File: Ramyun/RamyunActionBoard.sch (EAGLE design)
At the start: 84 parts, among them Q1 BC817-16LT1SMD, Q2 BC817-16LT1SMD, Q3 NVF6P02, U1 MAX31856_ADAFRUIT, U10 PVN012PBF, U11 PVN012PBF, U12 PVN012PBF, U13 PVN012PBF, U2 MAX31856_ADAFRUIT, U3 NL17SZ17DFT, U4 GPS_ADAFRUIT, U5 BUZZER, U6 PVN012PBF, U7 PVN012PBF, U8 PVN012PBF, U9 PVN012PBF, X1 5267-03, X10 5267-02, X11 5267-02, X12 5267-02, X13 5267-02, X14 5267-02, X15 5267-02, X16 5267-02, X2 5267-03, X3 5267-03, X4 USB+SHIELD, X5 5267-02, X6 5267-02, X7 5267-02, X8 5267-02, X9 5267-02

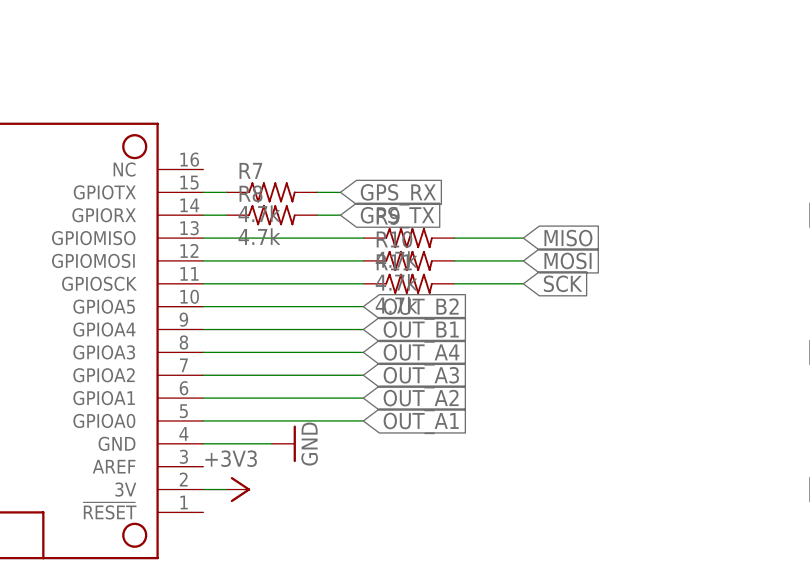
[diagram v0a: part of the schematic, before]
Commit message: value changed
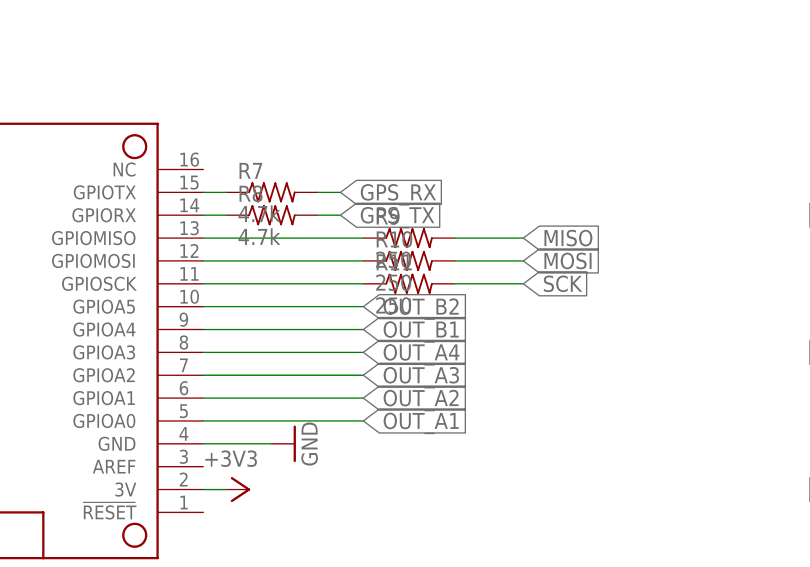
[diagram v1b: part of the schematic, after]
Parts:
- R10, R11, R9: value 4.7k -> 250
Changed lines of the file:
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@@
 <part name="GND_EXT25" library="GFE" deviceset="GND_EXT2" device=""/>
 <part name="GND25" library="GFE" deviceset="GND" device=""/>
-<part name="R9" library="GFE" deviceset="R" device="0603(1608)_HAND" value="4.7k"/>
-<part name="R10" library="GFE" deviceset="R" device="0603(1608)_HAND" value="4.7k"/>
-<part name="R11" library="GFE" deviceset="R" device="0603(1608)_HAND" value="4.7k"/>
+<part name="R9" library="GFE" deviceset="R" device="0603(1608)_HAND" value="250"/>
+<part name="R10" library="GFE" deviceset="R" device="0603(1608)_HAND" value="250"/>
+<part name="R11" library="GFE" deviceset="R" device="0603(1608)_HAND" value="250"/>
 <part name="+3V31" library="supply1" deviceset="+3V3" device=""/>
 <part name="+3V32" library="supply1" deviceset="+3V3" device=""/>

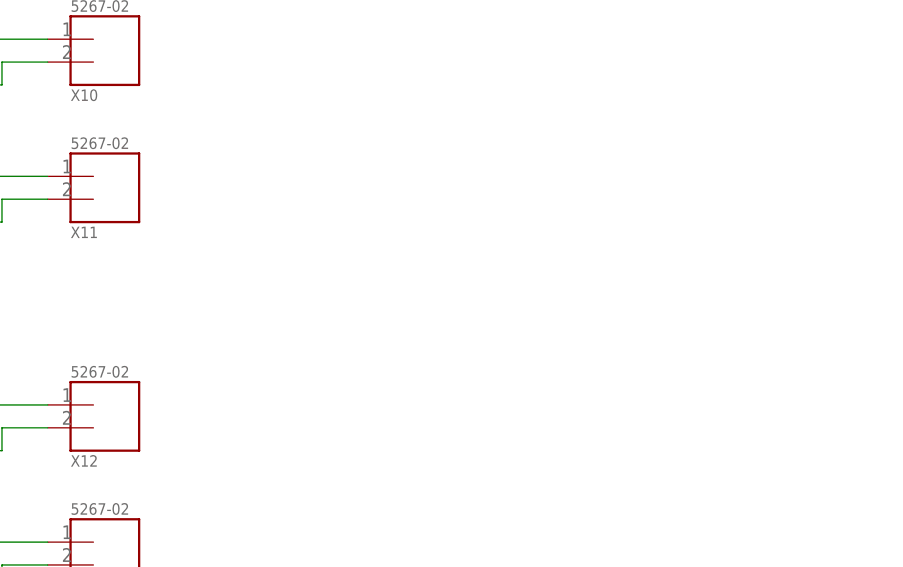
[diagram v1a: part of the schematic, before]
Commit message: duck
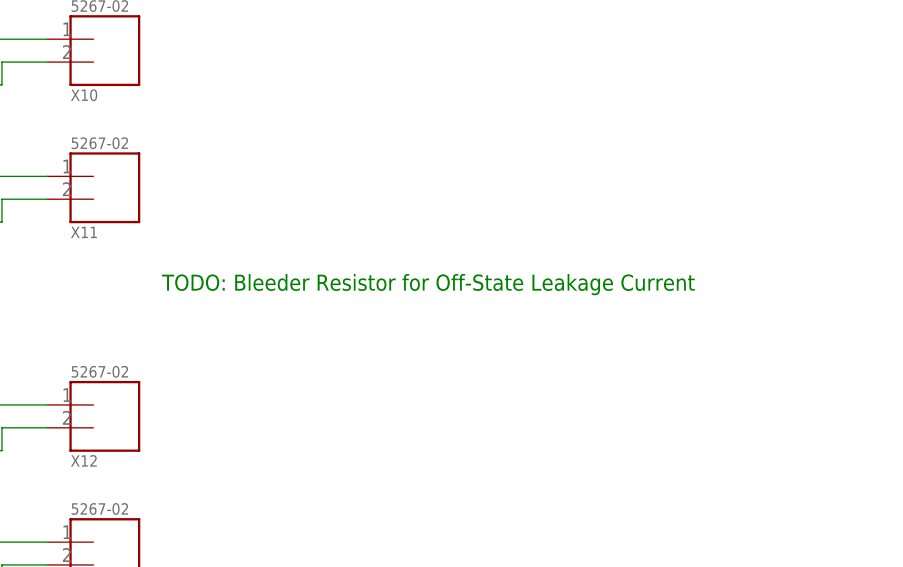
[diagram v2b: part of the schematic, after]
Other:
- note added: "TODO: Bleeder Resistor for Off-State Leakage Current"
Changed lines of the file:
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@@
 <text x="172.72" y="213.36" size="1.778" layer="91">5V reverse voltage protection</text>
 <text x="53.34" y="88.9" size="1.778" layer="91">TODO: solve USB power back-feeding!!</text>
+<text x="302.26" y="147.32" size="1.778" layer="91">TODO: Bleeder Resistor for Off-State Leakage Current </text>
 </plain>
 <instances>
